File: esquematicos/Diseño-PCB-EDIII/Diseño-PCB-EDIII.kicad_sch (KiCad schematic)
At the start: 34 parts, among them J1 Alimentación - Fuente +5V, J2 SerialToUSB-Converter, J4 OPT101, J5 Alimentación - Fuente +12V, J6 LAMPARA 12V, Q1 Q_NPN_BCE, Q2 Q_NPN_BCE, Q3 Q_NPN_BCE, Q4 Q_NPN_BCE, Q6 NMOS, SW1 ON/OFF, U2 SC39-11EWA, U3 SC39-11EWA, U4 SC39-11EWA, U5 SC39-11EWA, U6 PC817

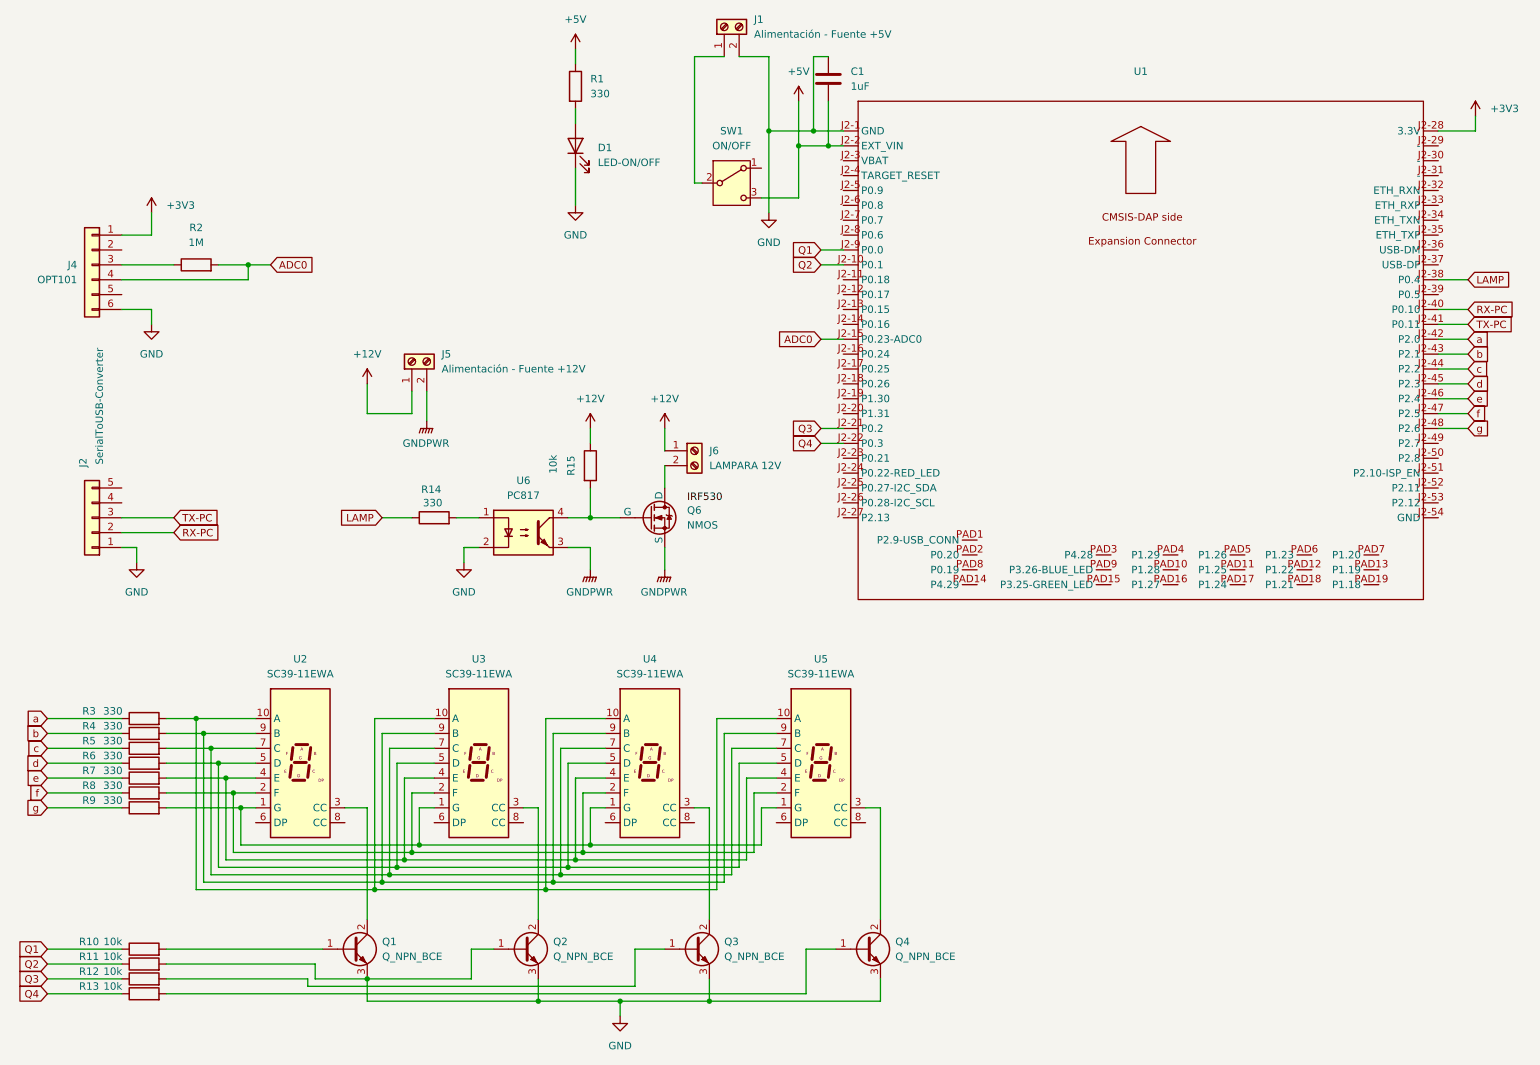
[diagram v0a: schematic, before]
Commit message: Version Funcionando + Interfaz grafica actualizada + adicionales para la calibracion
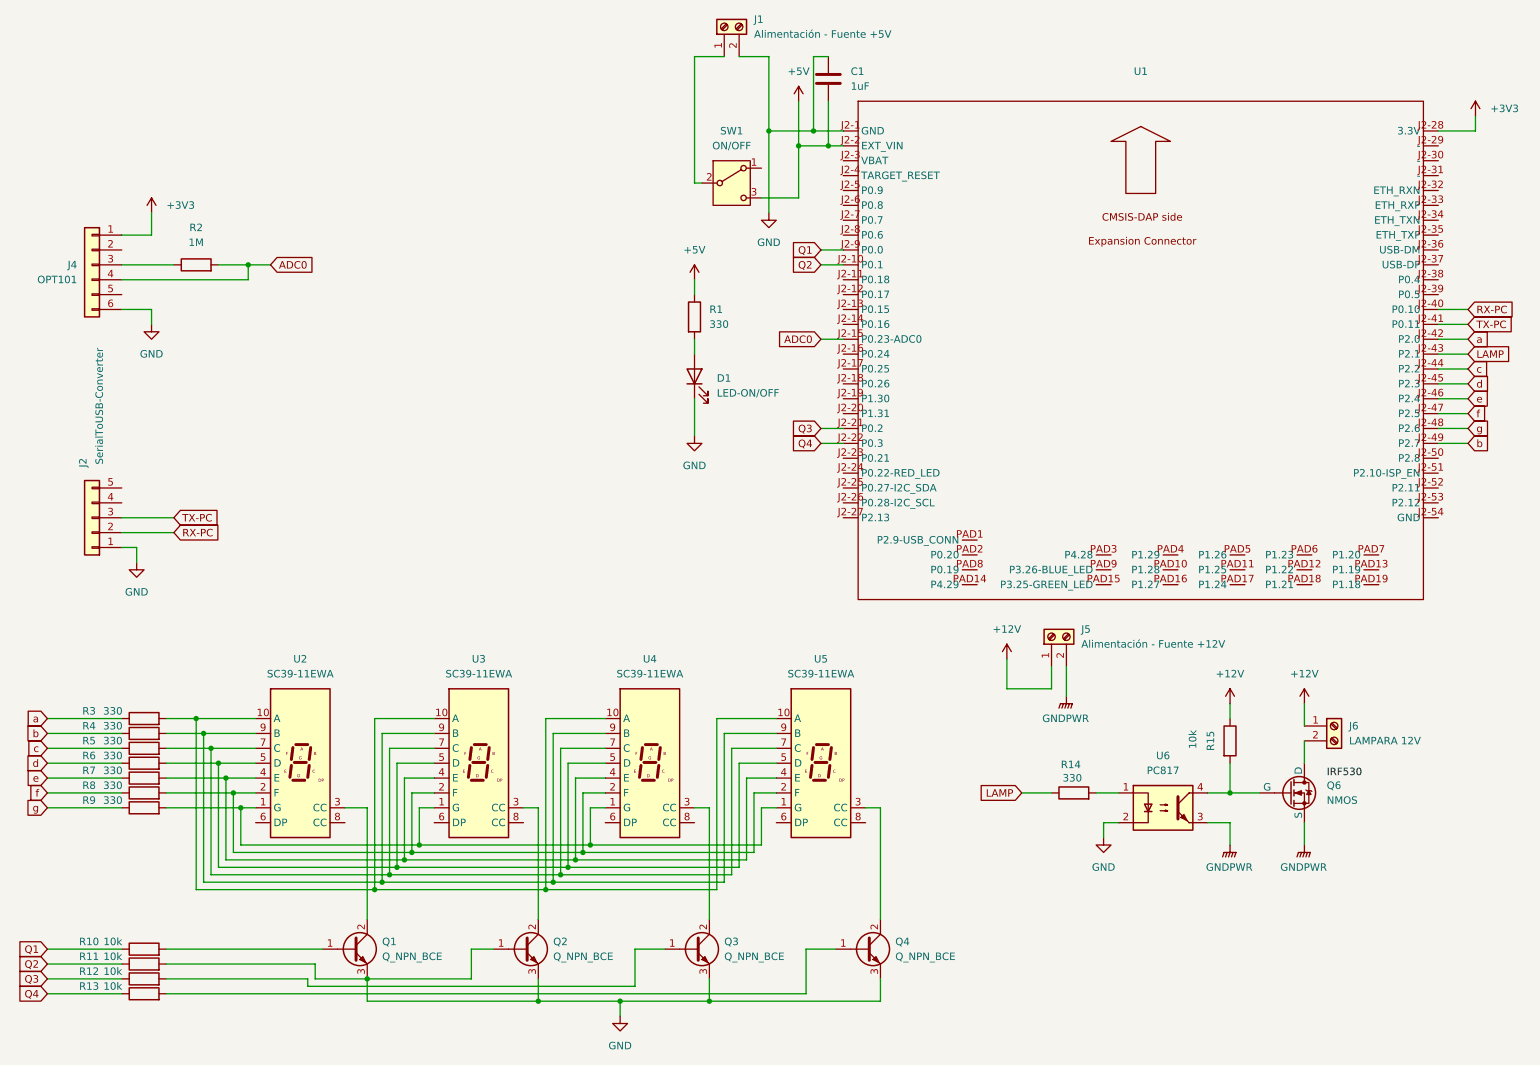
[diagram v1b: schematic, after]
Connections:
- net LAMP: now also U1.J2-43 (P2.1); no longer U1.J2-38 (P0.4)
- net b: now also U1.J2-49 (P2.7); no longer U1.J2-43 (P2.1)
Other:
- moved on the sheet: D1, J5, J6, Q6, R1, R14, R15, U6
